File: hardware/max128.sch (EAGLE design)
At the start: 11 parts, among them IC1 REG1117, IC2 EPM7128-P100, U2 AY-3-8910, X1 SCART-F

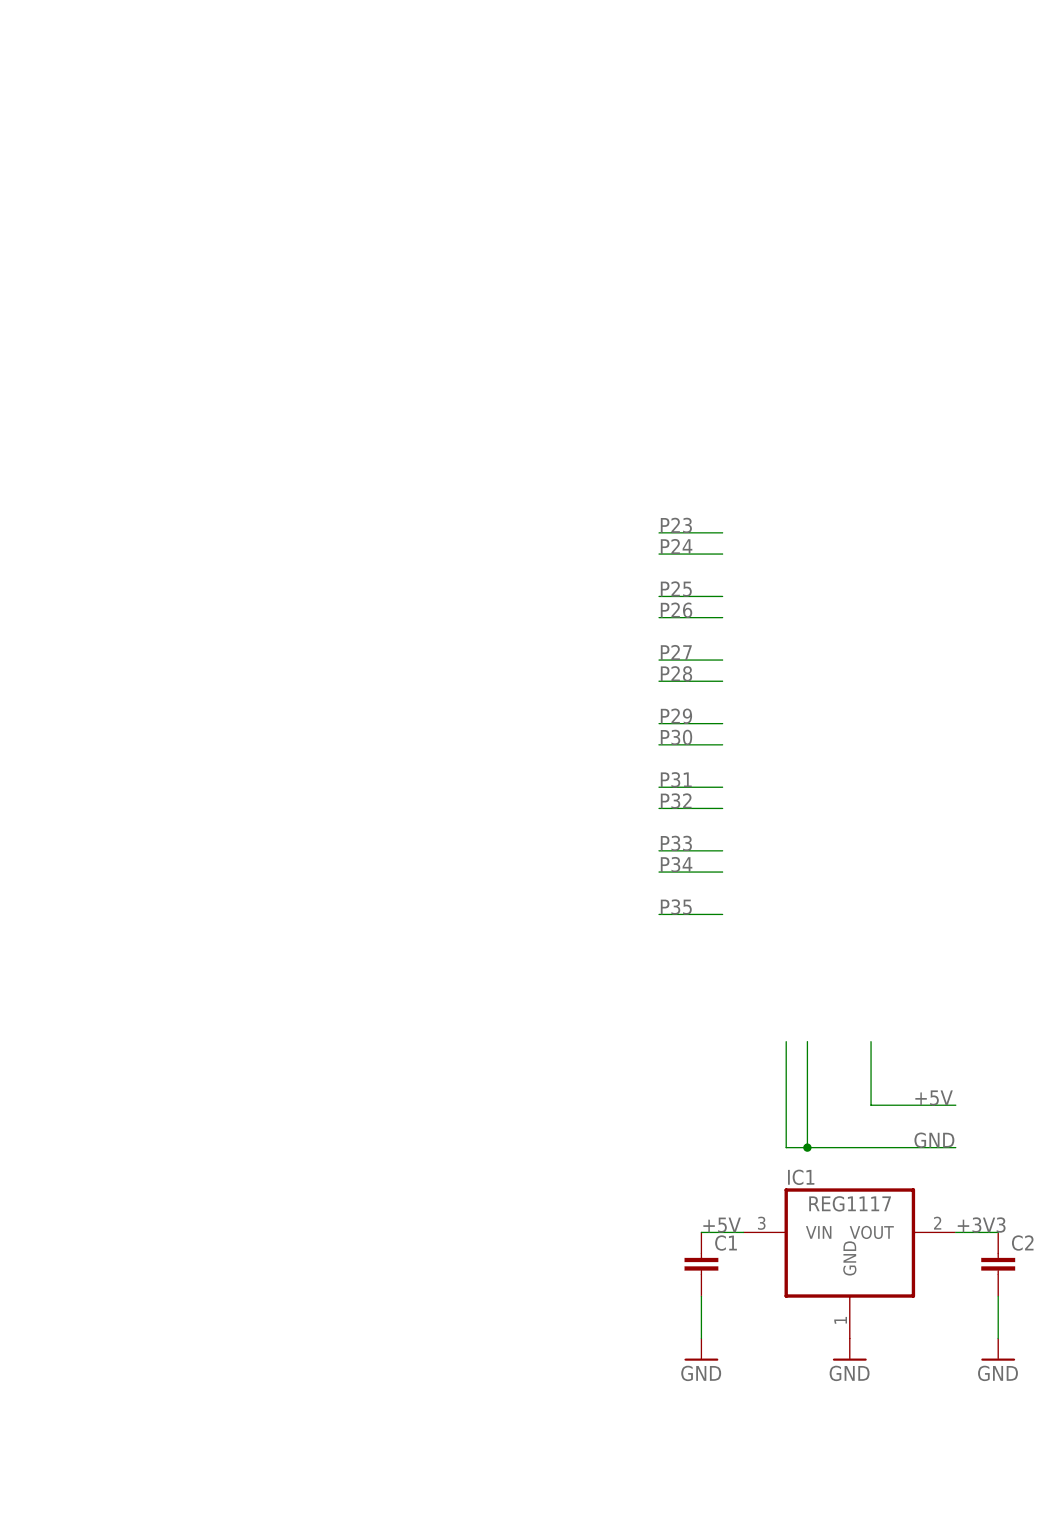
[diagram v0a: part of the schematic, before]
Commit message: Añado cambios
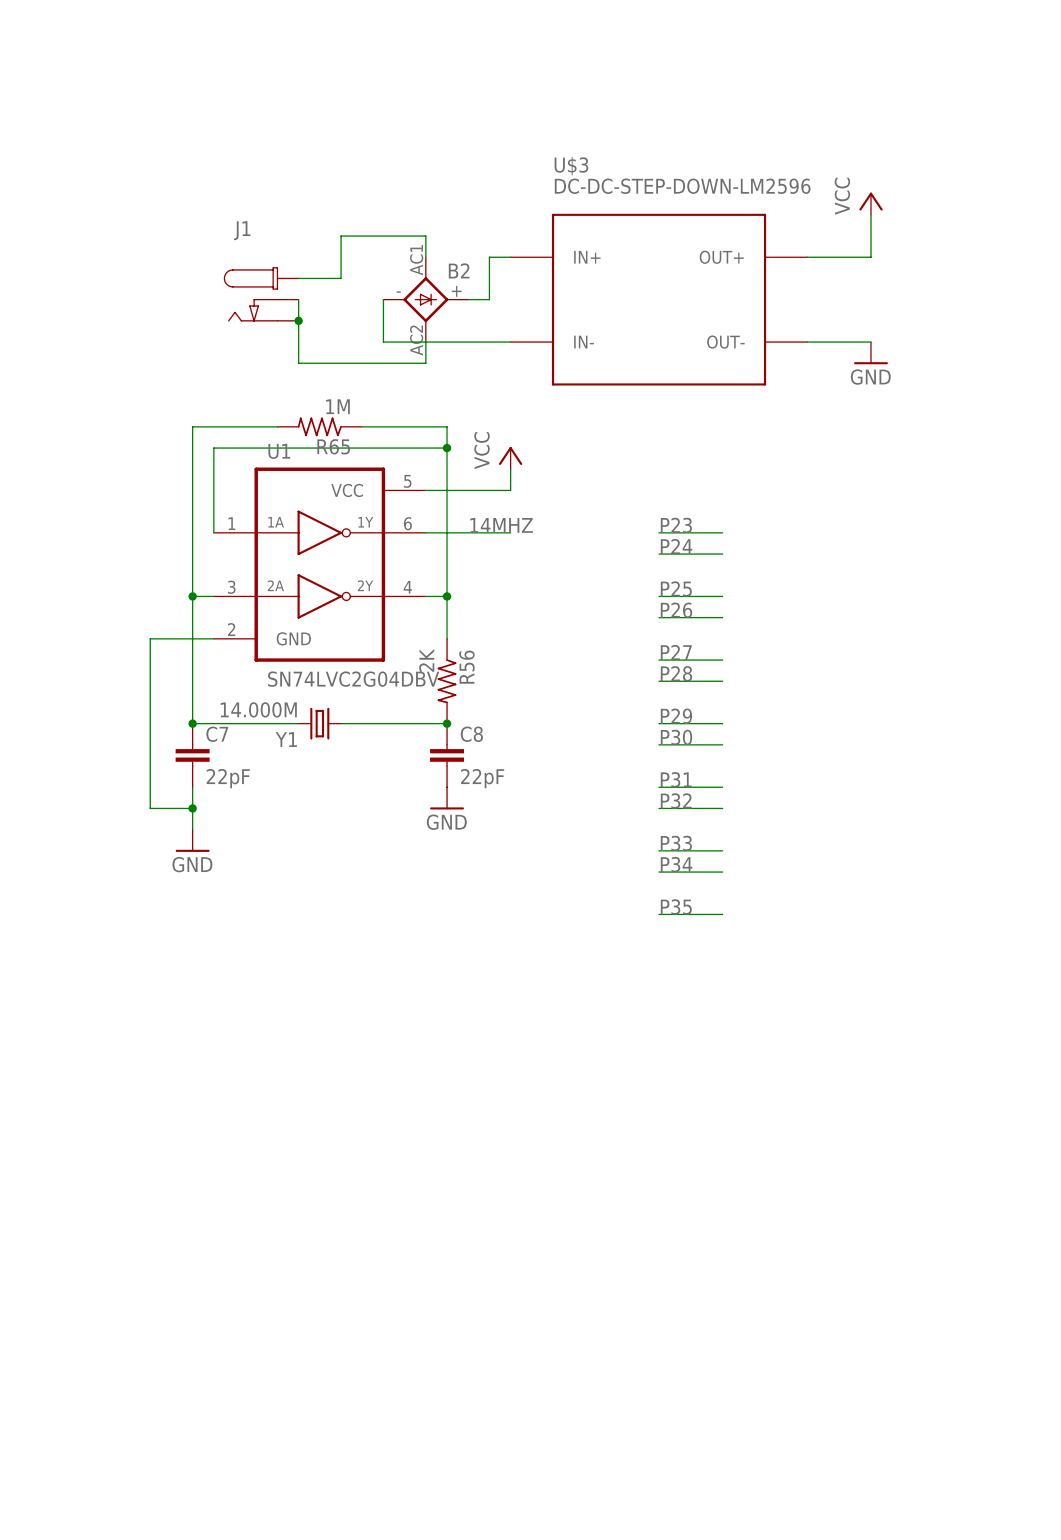
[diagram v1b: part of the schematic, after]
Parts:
- removed C1, C2: (no value), rcl:C-EUC0805
- removed IC1: REG1117, burr-brown:REG1117
- added B2: (no value), rectifier:1KAB
- added C7, C8: 22pF, rcl:C-EUC0805K
- added J1: (no value), dp_devices:CON_DC_M-DC_PTH2
- added R56: 2K, rcl:R-US_R0805
- added R65: 1M, rcl:R-US_R0805
- added U$3: DC-DC-STEP-DOWN-LM2596, diy-modules:DC-DC-STEP-DOWN-LM2596
- added U1: SN74LVC2G04DBV, 74LV:SN74LVC2G04DBV
- added Y1: 14.000M, crystal:CRYSTALHC49S
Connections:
- removed net +3V3: C2.1, IC1.VOUT
- new net 14MHZ: U1.1Y
- new net N$1: B2.AC1, J1.P1
- new net N$2: B2.AC2, J1.P2, J1.P3
- new net N$24: C7.1, R65.2, U1.2A, Y1.2
- new net N$27: R56.1, R65.1, U1.1A, U1.2Y
- new net N$3: B2.+, U$3.IN+
- new net N$4: B2.-, U$3.IN-
- new net N$61: C8.1, R56.2, Y1.1
- new net VCC: U$3.OUT+, U1.VCC
- net +5V: no longer C1.1, IC1.VIN
- net GND: now also C7.2, C8.2, U$3.OUT-, U1.GND; no longer C1.2, C2.2, IC1.GND
